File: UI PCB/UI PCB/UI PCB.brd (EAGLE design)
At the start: 88.9 x 74.6 mm, 23 parts, among them IC1 MCP23S17SP, IC2 MCP23S17SP, X1 JST-XH-02-PIN-ROUND-PAD, X2 JST-XH-02-PIN-ROUND-PAD, X3 JST-XH-02-PIN-ROUND-PAD, X4 JST-XH-02-PIN-ROUND-PAD, X5 JST-XH-05-PIN-ROUND-PAD, X6 JST-XH-05-PIN-ROUND-PAD, X7 JST-XH-05-PIN-ROUND-PAD, X8 JST-XH-05-PIN-ROUND-PAD, X9 JST-XH-05-PIN-ROUND-PAD

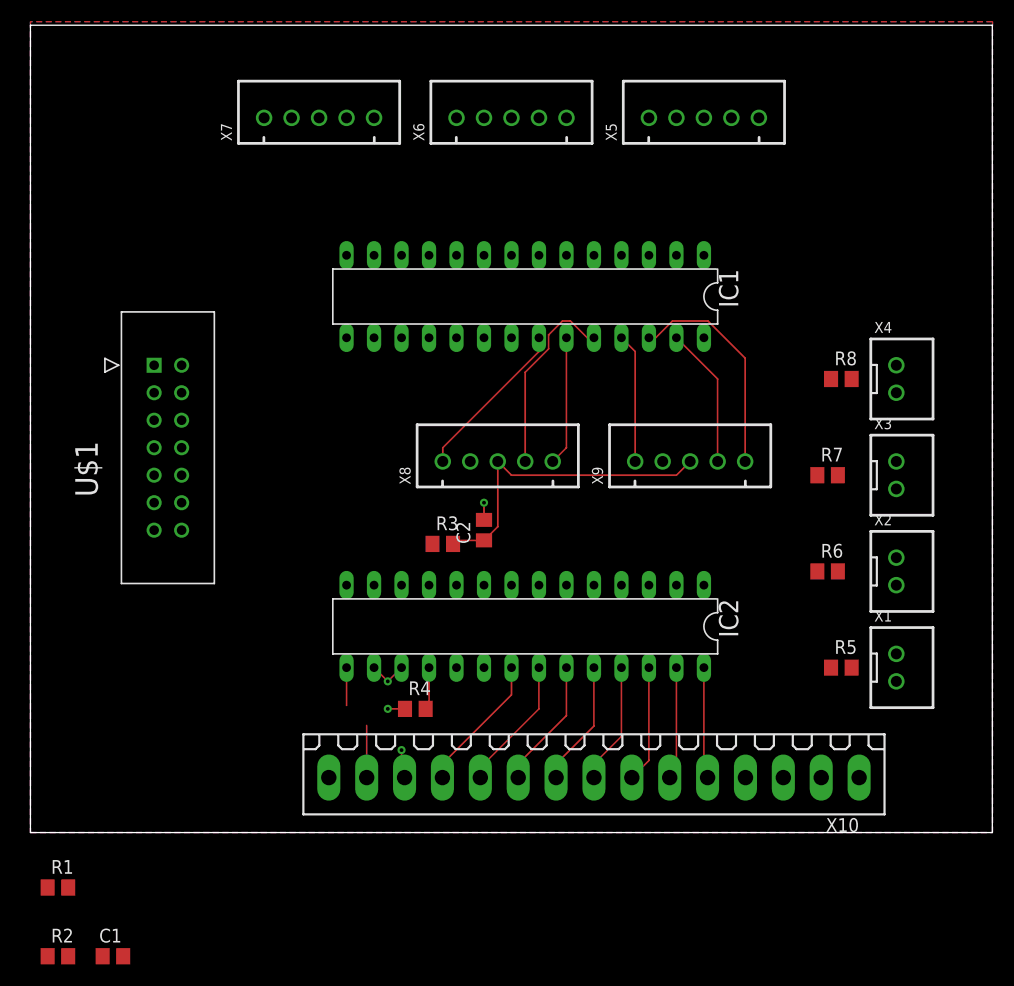
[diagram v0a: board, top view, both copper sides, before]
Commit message: redesigned PCB
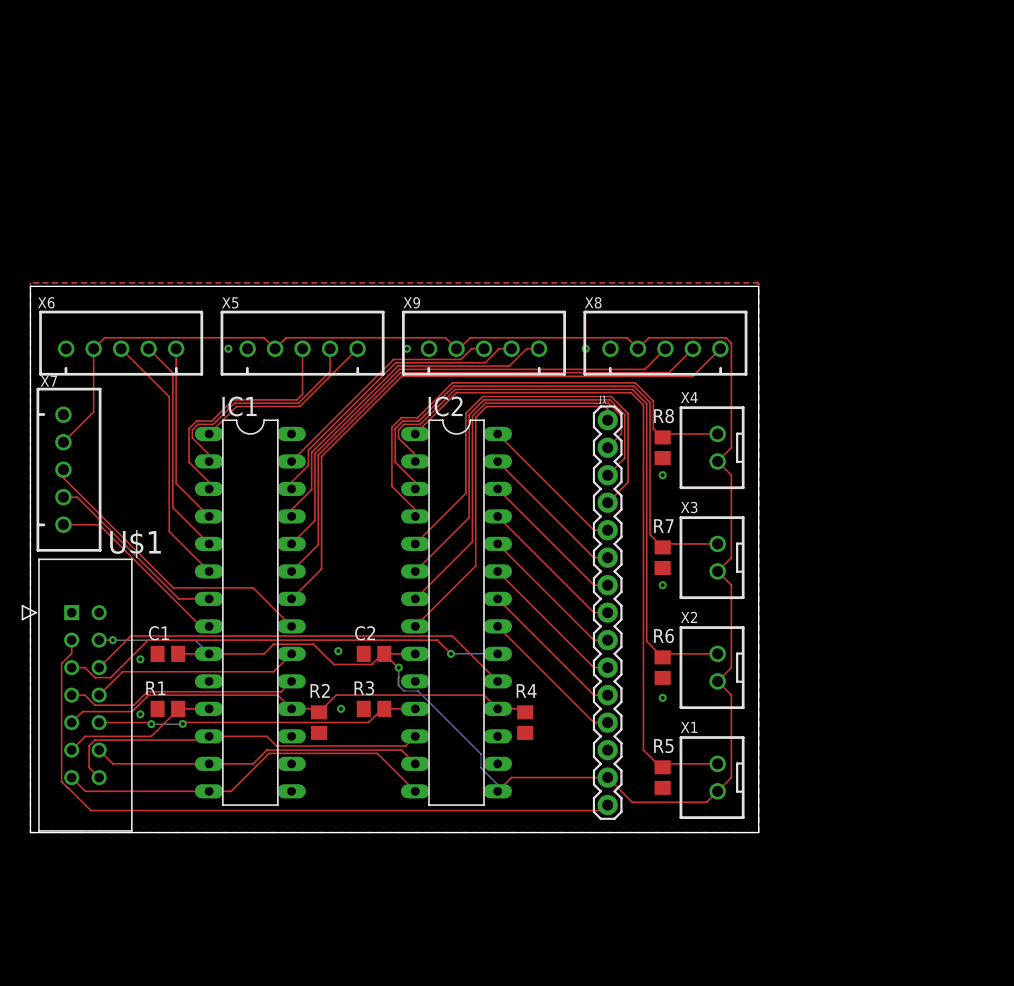
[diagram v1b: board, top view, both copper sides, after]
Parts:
- removed X10: (no value), con-weidmueller-sl35:180G-15
- added J1: (no value), SparkFun-Connectors:1X15
- moved X5 42.8 mm to (25.1, 44.7)
- moved X6 41.9 mm to (8.38, 44.7)
- moved X7 40.2 mm to (3.05, 33.5), turned to 270 degrees
- moved IC1 38.7 mm to (20.3, 20.3), turned to 270 degrees
- moved R2 32.4 mm to (26.7, 10.2), turned to 90 degrees
- moved C1 28.4 mm to (12.7, 16.5), turned to 180 degrees
- moved U$1 24.1 mm to (6.35, 20.3)
- moved X9 21.7 mm to (41.9, 44.7)
- moved R5 19.4 mm to (58.4, 5.08), turned to 90 degrees
- moved X1 19.4 mm to (63.5, 5.08), turned to 90 degrees
- moved R1 19.4 mm to (12.7, 11.4)
- moved X2 18.8 mm to (63.5, 15.2), turned to 90 degrees
- moved X8 18.7 mm to (58.7, 44.7)
- moved X3 18.2 mm to (63.5, 25.4), turned to 90 degrees
- moved R8 17.7 mm to (58.4, 35.6), turned to 90 degrees
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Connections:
- net 3V3: now also J1.14, X5.2, X6.2, X7.2, X8.2, X9.2; no longer X10.14, X5.3, X6.3, X7.3, X8.3, X9.3
- net 5V: now also J1.15; no longer X10.15
- net GND: now also J1.13, X5.1, X6.1, X7.1, X8.1, X9.1; no longer X10.13, X5.2, X6.2, X7.2, X8.2, X9.2
- net GPA0: now also J1.12; no longer X10.12
- net GPA1: now also J1.11; no longer X10.11
- net GPA2: now also J1.10; no longer X10.10
- net GPA3: now also J1.9; no longer X10.9
- net GPA4: now also J1.8; no longer X10.8
- net GPA5: now also J1.7; no longer X10.7
- net GPA6: now also J1.6; no longer X10.6
- net GPA7: now also J1.5; no longer X10.5
- net GPB4: now also J1.4; no longer X10.4
- net GPB5: now also J1.3; no longer X10.3
- net GPB6: now also J1.2; no longer X10.2
- net GPB7: now also J1.1; no longer X10.1
- net ROTARY_ENC_1_A: now also X5.5; no longer X5.1
- net ROTARY_ENC_1_B: now also X5.4; no longer X5.5
- net ROTARY_ENC_1_BUTTON: now also X5.3; no longer X5.4
- net ROTARY_ENC_2_A: now also X6.5; no longer X6.1
- net ROTARY_ENC_2_B: now also X6.4; no longer X6.5
- net ROTARY_ENC_2_BUTTON: now also X6.3; no longer X6.4
- net ROTARY_ENC_3_A: now also IC1.8, X7.5; no longer IC1.7, X7.1
- net ROTARY_ENC_3_B: now also IC1.7, X7.4; no longer IC1.8, X7.5
- net ROTARY_ENC_3_BUTTON: now also X7.3; no longer X7.4
- net ROTARY_ENC_4_A: now also X8.5; no longer X8.1
- net ROTARY_ENC_4_B: now also X8.4; no longer X8.5
- net ROTARY_ENC_4_BUTTON: now also X8.3; no longer X8.4
- net ROTARY_ENC_5_A: now also X9.5; no longer X9.1
- net ROTARY_ENC_5_B: now also X9.4; no longer X9.5
- net ROTARY_ENC_5_BUTTON: now also X9.3; no longer X9.4
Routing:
- net 3V3: track 37.5 -> 191.2 mm, vias 0 -> 2
- net 5V: track 0.00 -> 65.2 mm
- net CS1_BUTTON: track 0.00 -> 62.7 mm
- net CS2_BUTTON: track 0.00 -> 57.8 mm
- net CS3_BUTTON: track 0.00 -> 51.2 mm
- net CS4_BUTTON: track 0.00 -> 44.7 mm
- net INTA2: track 0.00 -> 41.7 mm, vias 0 -> 1
- net RESET: track 3.94 -> 44.9 mm
- net ROTARY_ENC_4_A: track 15.1 -> 55.3 mm
- net INTB2: track 0.00 -> 39.8 mm
- net GPB4: track 0.00 -> 39.3 mm
- net ROTARY_ENC_4_B: track 12.0 -> 50.5 mm
- net GPB5: track 0.00 -> 38.3 mm
- net GPB6: track 0.00 -> 37.3 mm
- net GPB7: track 0.00 -> 35.4 mm
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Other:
- board size 88.9 x 74.6 mm -> 67.3 x 50.5 mm
